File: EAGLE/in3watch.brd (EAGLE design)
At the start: 297 parts, among them IC1 74HC595D, IC2 74HC595D, IC3 74HC595D, IC4 74HC595D, IC5 74HC595D, IC6 74HC595D, IC7 74HC595D, J3 J5MM

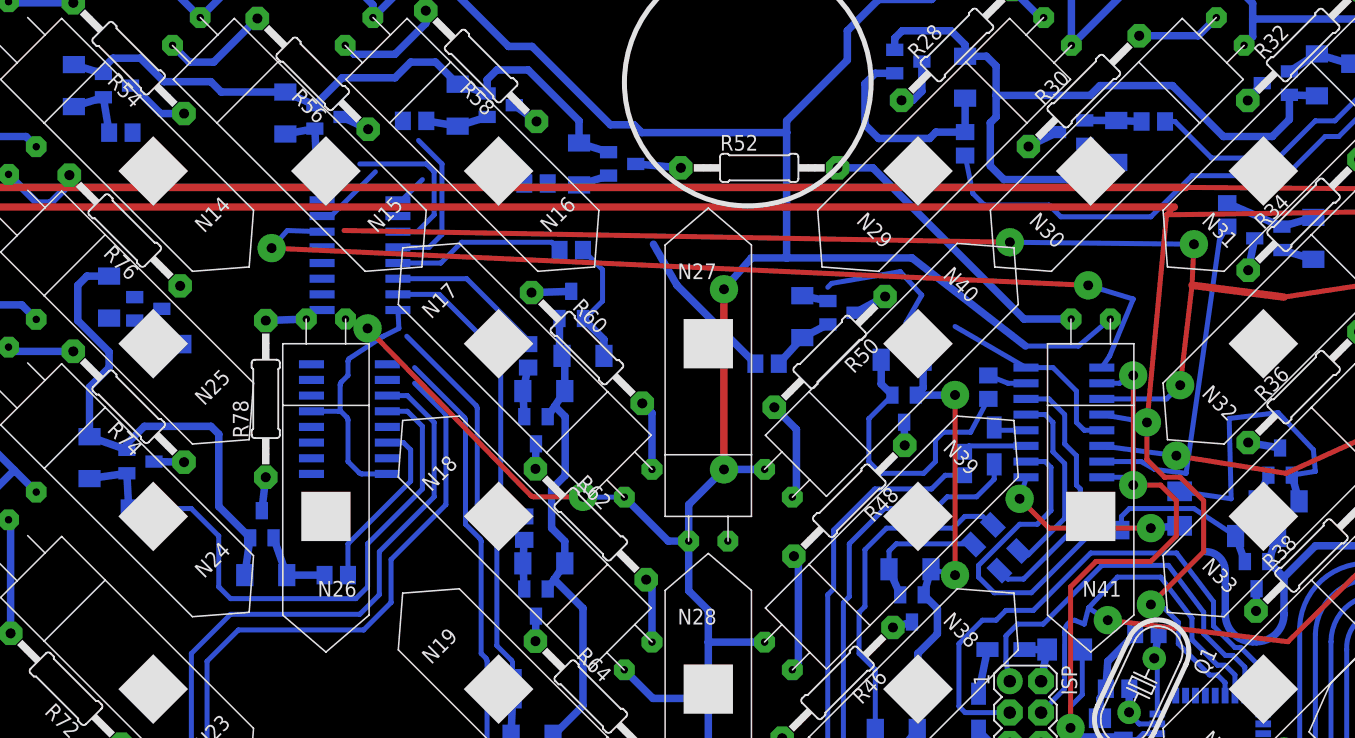
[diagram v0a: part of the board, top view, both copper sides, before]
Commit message: ..
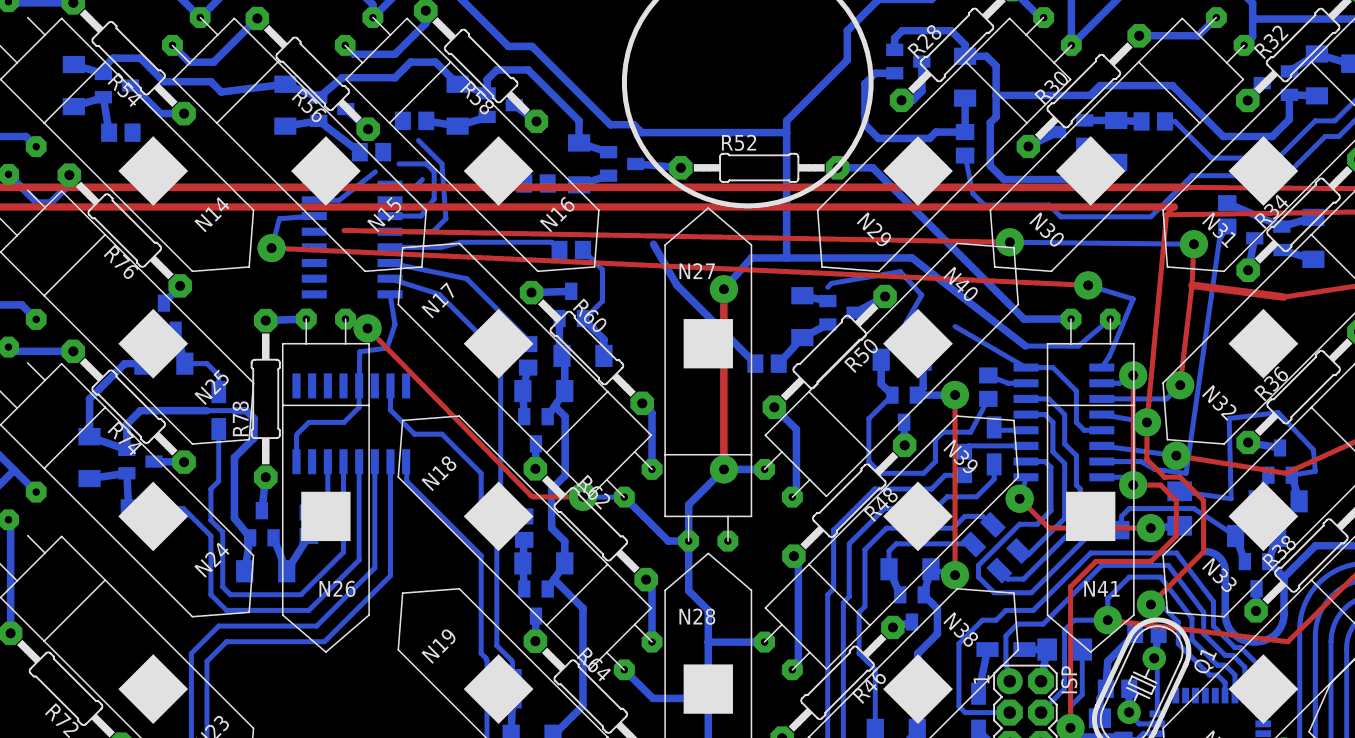
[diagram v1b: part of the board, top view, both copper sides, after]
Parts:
- R75: device rcl:R0805 -> rcl:R1206W
- moved VD38 6.99 mm to (-44.1, 12.4), turned to 0 degrees
- moved R75 6.61 mm to (-39.7, 8.57), turned to 90 degrees
- moved R77 4.69 mm to (-32.4, -0.64), turned to 270 degrees
- moved R55 3.72 mm to (-27.3, 29.5)
- moved VT38 1.42 mm to (-44.1, 16.2), turned to 0 degrees
- moved IC4 1.42 mm to (-28.9, 22.4)
- moved VT28 0.71 mm to (-30.5, 33.0)
- moved VD28 0.63 mm to (-34.3, 33.3)
- moved IC5 0.41 mm to (-28.9, 7.51), turned to 0 degrees
- moved VD39 0.32 mm to (-35.9, -4.45)
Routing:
- net RC12: track 0.00 -> 32.3 mm
- net RC10: track 50.1 -> 38.7 mm
- net RC9: track 57.3 -> 46.7 mm
- net RC13: track 14.4 -> 4.76 mm
- net RC11: track 41.5 -> 32.7 mm
- net N$83: track 0.00 -> 7.31 mm
- net RC8: track 39.4 -> 32.1 mm
- net RC2: track 13.3 -> 9.59 mm
- net RC7: track 31.1 -> 29.0 mm
- net N$82: track 0.00 -> 1.92 mm
- net RDATA_MOSI_D11: track 109.5 -> 108.1 mm
- net N$59: track 5.61 -> 6.93 mm
- net GND: track 1393.6 -> 1394.8 mm
- net RC6: track 24.2 -> 25.0 mm
- net RC5: track 12.9 -> 13.7 mm
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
